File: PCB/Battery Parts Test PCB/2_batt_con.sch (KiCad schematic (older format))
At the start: 27 parts, among them P4 CONN_7, Q10 MOSFET_N/NDS7002A, Q11 MOSFET_N/NDS7002A, Q12 MOSFET_N/NDS7002A, Q7 MOSFET_N/NDS7002A, Q8 MOSFET_N/NDS7002A, Q9 MOSFET_N/NDS7002A

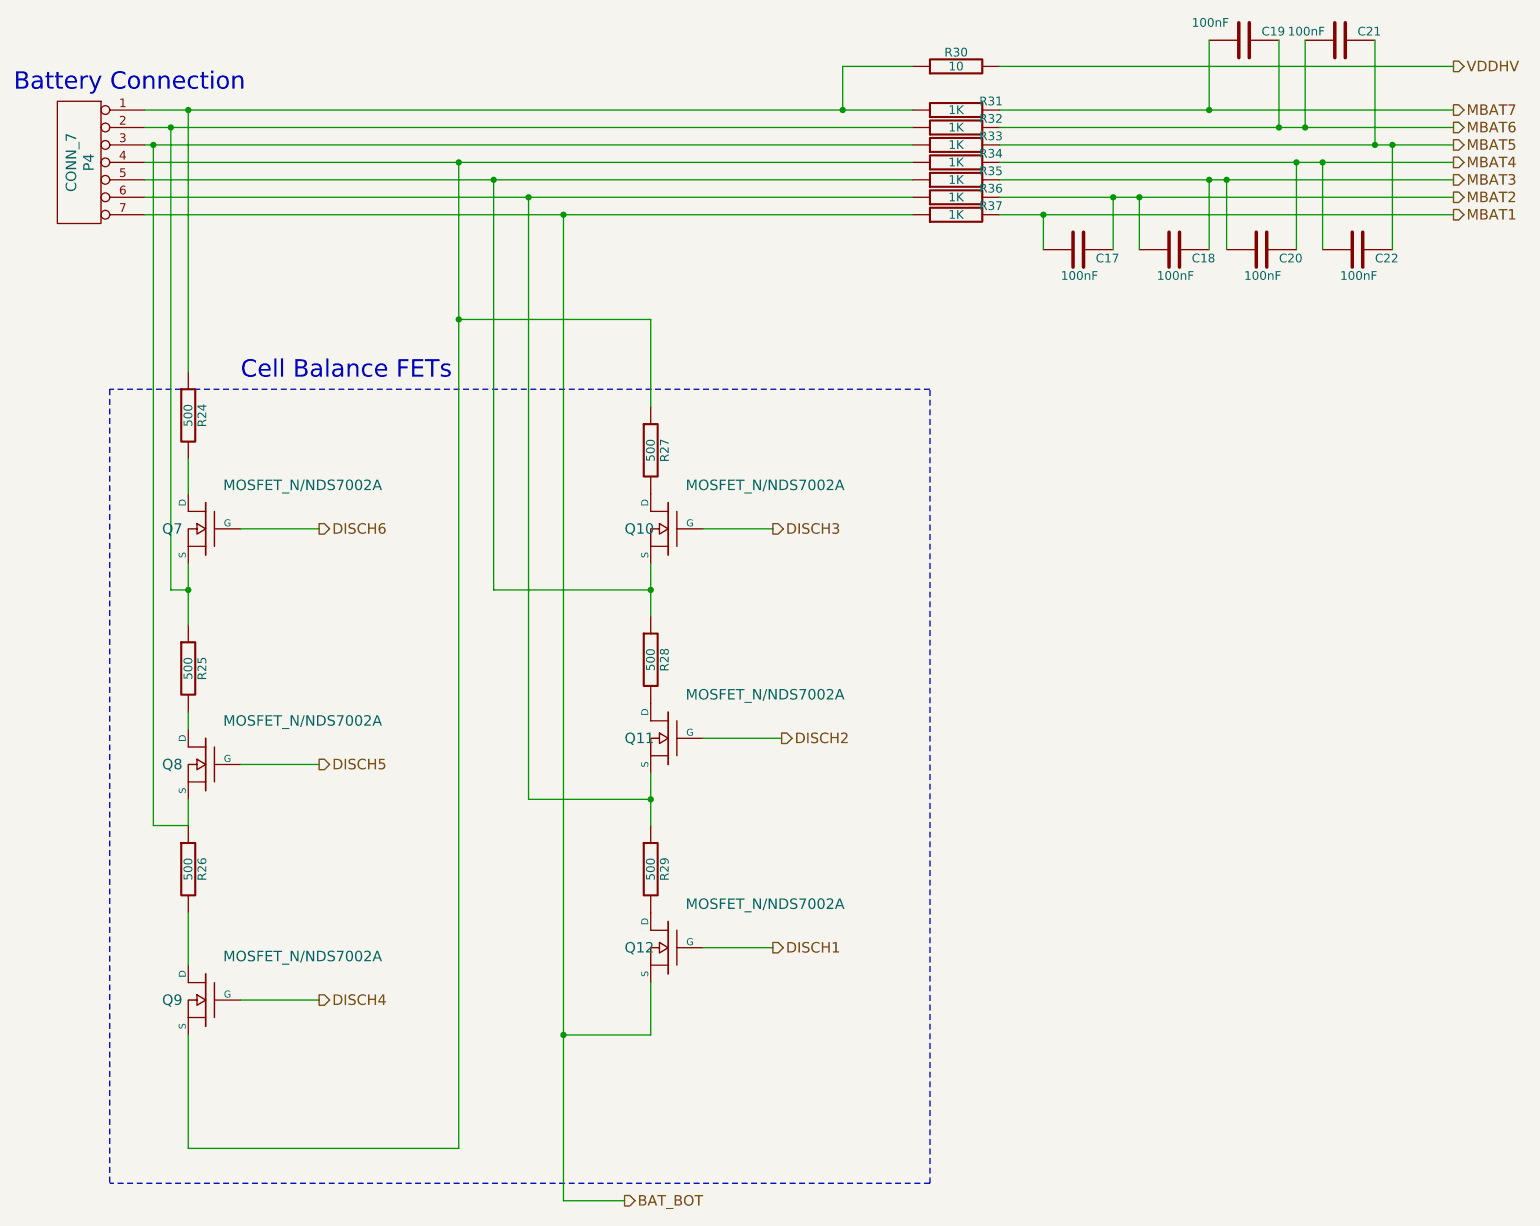
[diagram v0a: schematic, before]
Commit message: updated schematic
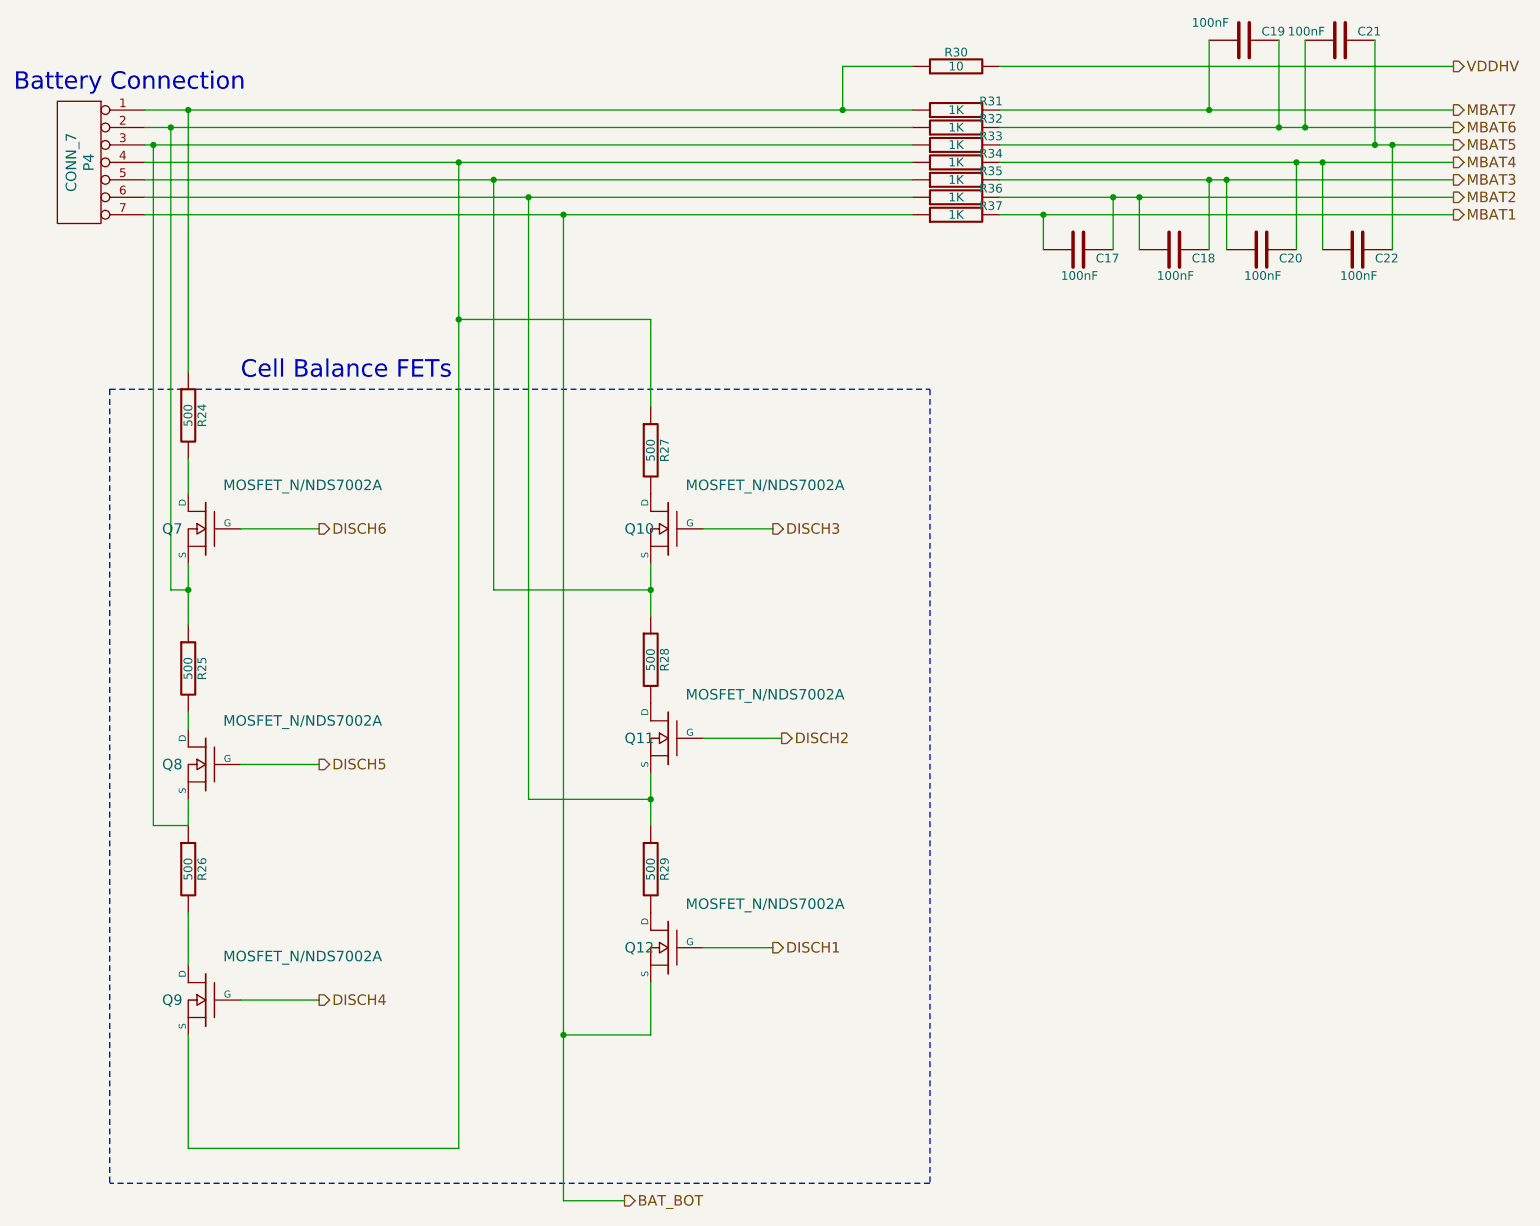
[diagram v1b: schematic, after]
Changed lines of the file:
@@
-EESchema Schematic File Version 2  date 4/30/2013 1:48:29 PM
+EESchema Schematic File Version 2  date 5/7/2013 3:13:49 PM
 LIBS:power
 LIBS:device
@@
 Sheet 8 9
 Title ""
-Date "30 apr 2013"
+Date "7 may 2013"
 Rev ""
 Comp ""
@@
 $EndComp
 Wire Wire Line
-	3700 7300 3700 1650
+	3700 1650 3700 7300
 Connection ~ 3700 6350
 Connection ~ 3500 1550
 Wire Wire Line
-	3500 5000 4200 5000
-Wire Wire Line
-	3500 1550 3500 5000
+	4200 5000 3500 5000
+Wire Wire Line
+	3500 5000 3500 1550
 Connection ~ 3100 2250
 Wire Wire Line
-	4200 2250 3100 2250
-Wire Wire Line
-	4200 2750 4200 2250
+	3100 2250 4200 2250
+Wire Wire Line
+	4200 2250 4200 2750
 Connection ~ 7800 1150
 Connection ~ 8350 1250
@@
 Connection ~ 3100 1350
 Wire Wire Line
-	3100 7000 3100 1350
-Wire Wire Line
-	1550 7000 3100 7000
+	3100 1350 3100 7000
+Wire Wire Line
+	3100 7000 1550 7000
 Wire Wire Line
 	4500 5850 4900 5850
@@
 	1850 3450 2300 3450
 Wire Wire Line
-	1350 5150 1350 1250
+	1350 1250 1350 5150
 Connection ~ 1550 3800
 Wire Wire Line
-	1450 3800 1550 3800
-Wire Wire Line
-	1450 1150 1450 3800
+	1550 3800 1450 3800
+Wire Wire Line
+	1450 3800 1450 1150
 Wire Wire Line
 	1550 2550 1550 1050
@@
 Connection ~ 5300 1050
 Wire Wire Line
-	5300 800  5300 1050
+	5300 1050 5300 800
 Wire Notes Line
 	1100 2650 1100 7200
@@
 Connection ~ 1350 1250
 Wire Wire Line
-	1550 5150 1550 5000
+	1550 5000 1550 5150
 Wire Wire Line
 	5700 1050 1300 1050
@@
 	4200 5150 4200 4850
 Wire Wire Line
-	4200 6350 4200 6050
-Wire Wire Line
-	5700 800  5300 800
+	4200 6050 4200 6350
+Wire Wire Line
+	5300 800  5700 800
 Wire Wire Line
 	1550 3050 1550 3250
@@
 	1550 5150 1350 5150
 Wire Wire Line
-	1550 6350 1550 7000
+	1550 7000 1550 6350
 Wire Wire Line
 	4500 4650 4950 4650
@@
 Connection ~ 7400 1050
 Wire Wire Line
-	3300 3800 3300 1450
-Wire Wire Line
-	4200 3800 3300 3800
+	3300 1450 3300 3800
+Wire Wire Line
+	3300 3800 4200 3800
 Connection ~ 3300 1450
 Wire Wire Line
-	3700 6350 4200 6350
+	4200 6350 3700 6350
 Connection ~ 3700 1650
 Wire Notes Line
-	5800 2650 1100 2650
+	1100 2650 5800 2650
 Wire Notes Line
-	5800 7200 5800 2650
+	5800 2650 5800 7200
 Wire Notes Line
 	5800 7200 1100 7200
 Wire Wire Line
-	4050 7300 3700 7300
+	3700 7300 4050 7300
 Text HLabel 4050 7300 2    60   Output ~ 0
 BAT_BOT
